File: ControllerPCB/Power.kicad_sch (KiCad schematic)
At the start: 9 parts, among them U1 ADP3336ARMZ, U3 TVS0500DRV

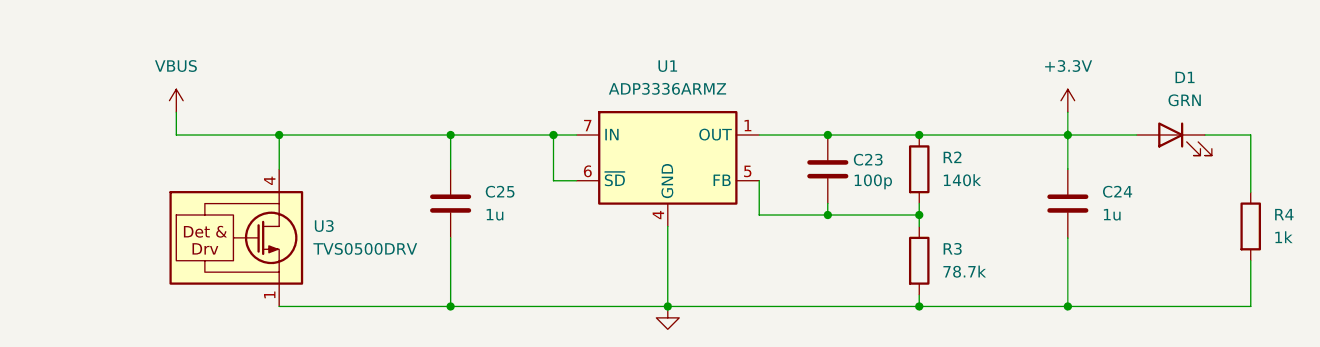
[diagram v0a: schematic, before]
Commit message: Updated many things.
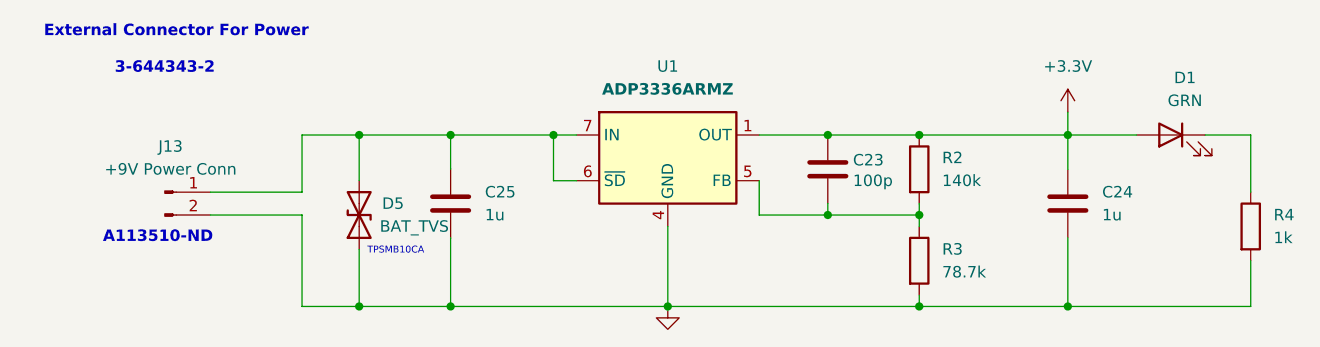
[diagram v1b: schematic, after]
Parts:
- removed U3: TVS0500DRV, Package_SON:WSON-6-1EP_2x2mm_P0.65mm_EP1x1.6mm, symbol Power_Protection:TVS0500DRV
- added D5: BAT_TVS, symbol Device:D_TVS
- added J13: +9V Power Conn, symbol Connector:Conn_01x02_Pin
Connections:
- net GND: now also D5.1 (A1), J13.2 (Pin_2)
- net VBUS: no longer names the net of C25.1, U1.6 (~{SD}), U1.7 (IN), U1.8 (IN)
- net VBUS: now also D5.2 (A2), J13.1 (Pin_1)
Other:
- note added: "3-644343-2"
- note added: "A113510-ND"
- note added: "External Connector For Power"
- note added: "TPSMB10CA"
